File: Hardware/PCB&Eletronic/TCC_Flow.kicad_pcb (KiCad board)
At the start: 2 copper layers, 147.3 x 68.6 mm, 42 parts, among them J1 ESP01, M3 MountingHole_3.2mm_M3, Q1 BC337, Q2 BC337, Q3 BC337, Q4 BC337

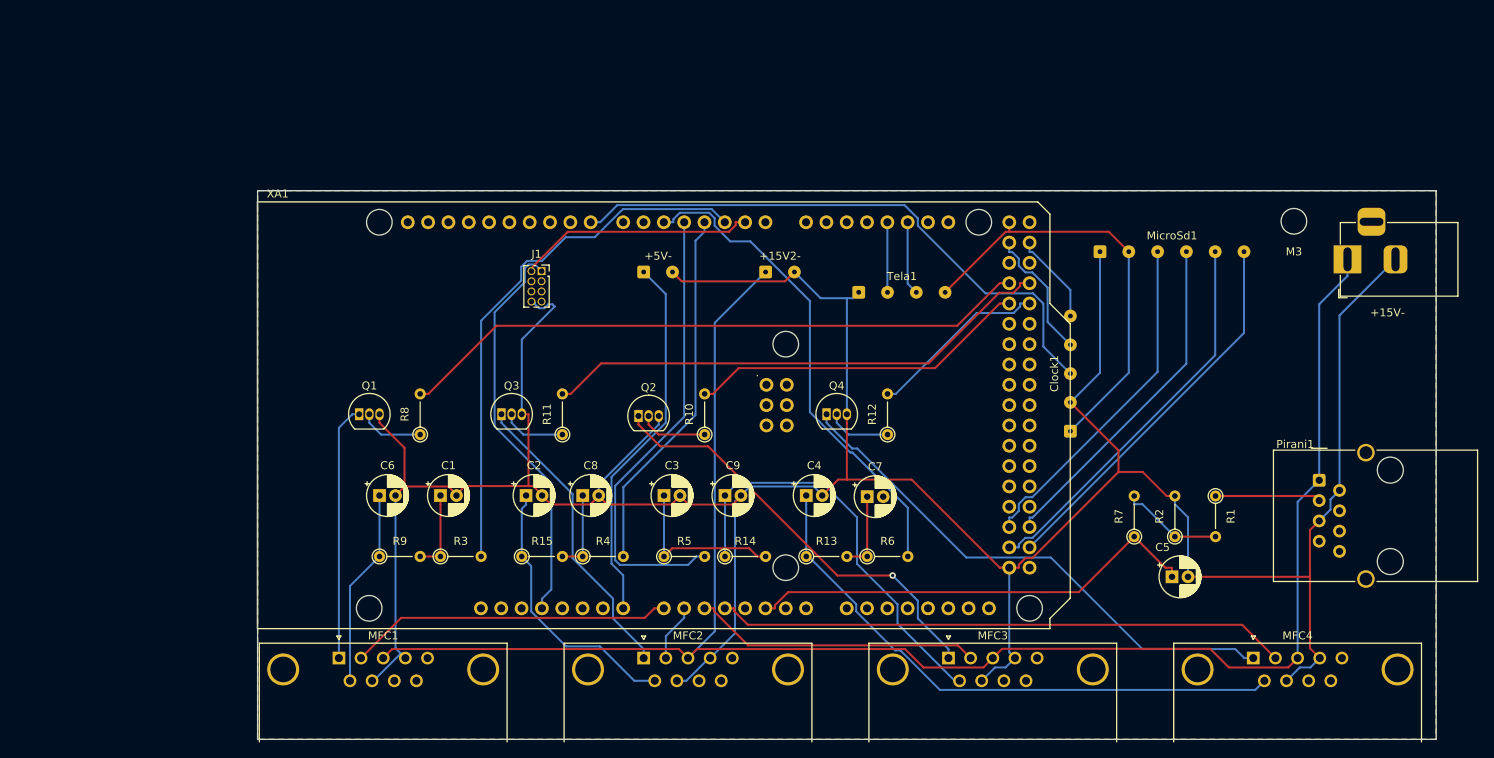
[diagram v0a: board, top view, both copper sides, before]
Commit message: [PCB] Add updated pcb and Doc
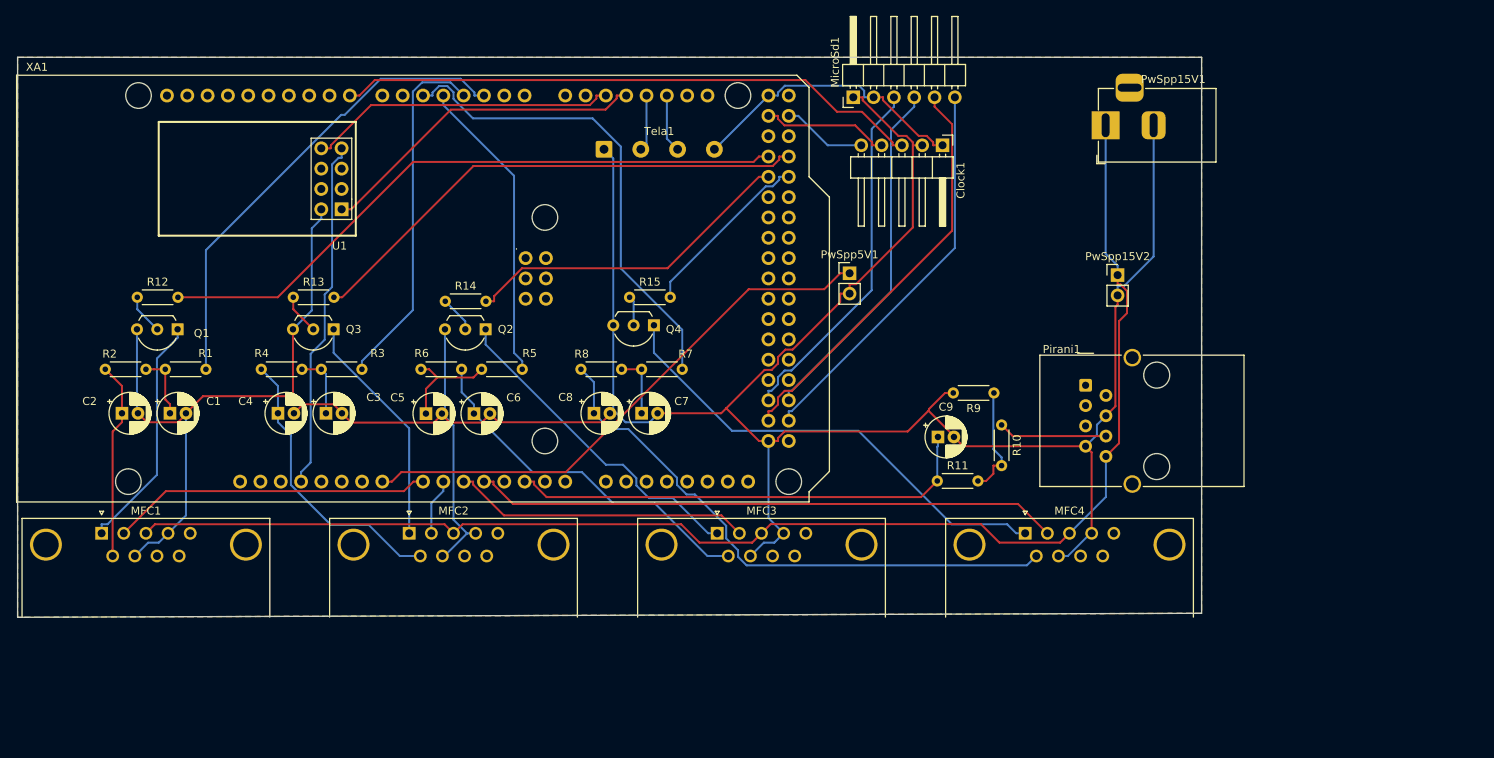
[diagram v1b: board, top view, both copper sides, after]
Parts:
- removed +15V-: Conn_01x02_Male, Connector_BarrelJack:BarrelJack_Horizontal
- removed +15V2-, +5V-: Conn_01x02_Male, Connector_Wire:SolderWire-0.1sqmm_1x02_P3.6mm_D0.4mm_OD1mm
- removed J1: ESP01, Connector_PinSocket_1.27mm:PinSocket_2x04_P1.27mm_Vertical
- removed M3: MountingHole_3.2mm_M3, MountingHole:MountingHole_3.2mm_M3
- added PwSpp15V1: Conn_01x02_Male, Connector_BarrelJack:BarrelJack_Horizontal, F.Cu at (169.5, 35.0)
- added PwSpp15V2: Conn_01x02_Male, Connector_PinHeader_2.54mm:PinHeader_1x02_P2.54mm_Vertical, F.Cu at (171.0, 53.7)
- added PwSpp5V1: Conn_01x02_Male, Connector_PinHeader_2.54mm:PinHeader_1x02_P2.54mm_Vertical, F.Cu at (137.5, 53.5)
- added U1: ESP-01v090, esp:ESP-01, F.Cu at (74.0, 45.5)
- Clock1: footprint Connector_Wire:SolderWire-0.1sqmm_1x05_P3.6mm_D0.4mm_OD1mm -> Connector_PinHeader_2.54mm:PinHeader_1x05_P2.54mm_Horizontal
- MicroSd1: footprint Connector_Wire:SolderWire-0.1sqmm_1x06_P3.6mm_D0.4mm_OD1mm -> Connector_PinHeader_2.54mm:PinHeader_1x06_P2.54mm_Horizontal
- Q1, Q2, Q3, Q4: footprint Package_TO_SOT_THT:TO-92_Inline -> Package_TO_SOT_THT:TO-92L_Inline_Wide
- R1, R2: value 4.6K -> 500; footprint Resistor_THT:R_Axial_DIN0204_L3.6mm_D1.6mm_P5.08mm_Vertical -> Resistor_THT:R_Axial_DIN0204_L3.6mm_D1.6mm_P5.08mm_Horizontal
- R10: value 4.7K -> 4.6K; footprint Resistor_THT:R_Axial_DIN0204_L3.6mm_D1.6mm_P5.08mm_Vertical -> Resistor_THT:R_Axial_DIN0204_L3.6mm_D1.6mm_P5.08mm_Horizontal
- R11: value 4.7K -> 220; footprint Resistor_THT:R_Axial_DIN0204_L3.6mm_D1.6mm_P5.08mm_Vertical -> Resistor_THT:R_Axial_DIN0204_L3.6mm_D1.6mm_P5.08mm_Horizontal
- R12: footprint Resistor_THT:R_Axial_DIN0204_L3.6mm_D1.6mm_P5.08mm_Vertical -> Resistor_THT:R_Axial_DIN0204_L3.6mm_D1.6mm_P5.08mm_Horizontal
- R13, R14, R15: value 1K -> 4.7K; footprint Resistor_THT:R_Axial_DIN0204_L3.6mm_D1.6mm_P5.08mm_Vertical -> Resistor_THT:R_Axial_DIN0204_L3.6mm_D1.6mm_P5.08mm_Horizontal
- R3, R4, R5, R6: value 1K -> 500; footprint Resistor_THT:R_Axial_DIN0204_L3.6mm_D1.6mm_P5.08mm_Vertical -> Resistor_THT:R_Axial_DIN0204_L3.6mm_D1.6mm_P5.08mm_Horizontal
- R7: value 220 -> 500; footprint Resistor_THT:R_Axial_DIN0204_L3.6mm_D1.6mm_P5.08mm_Vertical -> Resistor_THT:R_Axial_DIN0204_L3.6mm_D1.6mm_P5.08mm_Horizontal
- R8: value 4.7K -> 500; footprint Resistor_THT:R_Axial_DIN0204_L3.6mm_D1.6mm_P5.08mm_Vertical -> Resistor_THT:R_Axial_DIN0204_L3.6mm_D1.6mm_P5.08mm_Horizontal
- R9: value 1K -> 4.6K; footprint Resistor_THT:R_Axial_DIN0204_L3.6mm_D1.6mm_P5.08mm_Vertical -> Resistor_THT:R_Axial_DIN0204_L3.6mm_D1.6mm_P5.08mm_Horizontal
- Tela1: footprint Connector_Wire:SolderWire-0.1sqmm_1x04_P3.6mm_D0.4mm_OD1mm -> Connector_Wire:SolderWire-0.5sqmm_1x04_P4.6mm_D0.9mm_OD2.1mm
- moved R2 135.3 mm to (44.5, 65.5), turned to 0 degrees
- moved R1 132.2 mm to (52.0, 65.5), turned to 0 degrees
- moved C5 95.5 mm to (84.5, 71.0)
- moved R12 95.3 mm to (48.5, 56.5), turned to 0 degrees
- moved R9 79.5 mm to (155.5, 68.5), turned to 180 degrees
- moved R13 71.8 mm to (68.0, 56.5)
- moved C4 66.8 mm to (66.0, 71.0)
- moved R7 65.0 mm to (111.5, 65.5), turned to 0 degrees
- moved R6 55.8 mm to (89.0, 65.5), turned to 180 degrees
- moved C2 51.6 mm to (46.5, 71.0)
- moved R14 47.3 mm to (87.0, 57.0)
- moved R11 47.2 mm to (148.5, 79.5), turned to 0 degrees
- moved R4 46.5 mm to (64.0, 65.5)
- moved C3 43.5 mm to (72.0, 71.0)
- moved Clock1 39.1 mm to (149.1, 37.5), turned to -90 degrees
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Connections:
- C1 pad 1: Net-(R3-Pad1) -> Net-(C1-Pad1)
- C2 pad 1: Net-(MFC2-Pad6) -> Net-(C2-Pad1)
- C3 pad 1: Net-(R5-Pad1) -> Net-(C3-Pad1)
- C4 pad 1: Net-(MFC4-Pad6) -> Net-(C4-Pad1)
- C7 pad 1: Net-(R6-Pad1) -> Net-(C7-Pad1)
- C7 pad 2: unconnected-(C7-Pad2) -> Net-(C1-Pad2)
- C8 pad 1: Net-(R4-Pad1) -> Net-(C8-Pad1)
- C9 pad 1: Net-(MFC3-Pad6) -> Net-(C9-Pad1)
- MFC1 pad 6: Net-(C6-Pad1) -> Net-(C2-Pad1)
- MFC2 pad 6: Net-(MFC2-Pad6) -> Net-(C4-Pad1)
- MFC3 pad 6: Net-(MFC3-Pad6) -> Net-(C6-Pad1)
- MFC4 pad 6: Net-(MFC4-Pad6) -> Net-(C8-Pad1)
- Pirani1 pad 1: Net-(MFC1-Pad3) -> unconnected-(Pirani1-Pad1)
- Pirani1 pad 2: Net-(C1-Pad2) -> unconnected-(Pirani1-Pad2)
- Pirani1 pad 3: Net-(Pirani1-Pad3) -> unconnected-(Pirani1-Pad3)
- Pirani1 pad 4: unconnected-(Pirani1-Pad4) -> Net-(C1-Pad2)
- Pirani1 pad 5: Net-(C1-Pad2) -> unconnected-(Pirani1-Pad5)
- Pirani1 pad 6: unconnected-(Pirani1-Pad6) -> Net-(Pirani1-Pad6)
- Pirani1 pad 7: unconnected-(Pirani1-Pad7) -> Net-(C1-Pad2)
- Pirani1 pad 8: unconnected-(Pirani1-Pad8) -> Net-(MFC1-Pad3)
- R1 pad 1: Net-(Pirani1-Pad3) -> Net-(C1-Pad1)
- R10 pad 1: Net-(Q2-Pad2) -> Net-(Pirani1-Pad6)
- R11 pad 1: Net-(Q3-Pad2) -> Net-(C9-Pad1)
- R11 pad 2: Net-(R11-Pad2) -> Net-(R10-Pad2)
- R12 pad 1: Net-(Q4-Pad2) -> Net-(Q1-Pad2)
- R12 pad 2: Net-(XA1-PadD29) -> Net-(R12-Pad2)
- R13 pad 1: Net-(MFC4-Pad6) -> Net-(Q3-Pad2)
- R13 pad 2: Net-(R6-Pad1) -> Net-(R13-Pad2)
- R14 pad 1: Net-(MFC3-Pad6) -> Net-(Q2-Pad2)
- R14 pad 2: Net-(R5-Pad1) -> Net-(R14-Pad2)
- R15 pad 1: Net-(MFC2-Pad6) -> Net-(Q4-Pad2)
- R15 pad 2: Net-(R4-Pad1) -> Net-(R15-Pad2)
- R2 pad 1: Net-(R1-Pad2) -> Net-(C2-Pad1)
- R2 pad 2: Net-(C1-Pad2) -> Net-(C1-Pad1)
- R3 pad 1: Net-(R3-Pad1) -> Net-(C3-Pad1)
- R4 pad 1: Net-(R4-Pad1) -> Net-(C4-Pad1)
- R4 pad 2: Net-(R4-Pad2) -> Net-(C3-Pad1)
- R5 pad 1: Net-(R5-Pad1) -> Net-(C5-Pad1)
- R6 pad 1: Net-(R6-Pad1) -> Net-(C6-Pad1)
- R6 pad 2: Net-(R6-Pad2) -> Net-(C5-Pad1)
- R7 pad 1: Net-(C5-Pad1) -> Net-(C7-Pad1)
- R7 pad 2: Net-(R1-Pad2) -> Net-(R7-Pad2)
- R8 pad 1: Net-(Q1-Pad2) -> Net-(C8-Pad1)
- R8 pad 2: Net-(R8-Pad2) -> Net-(C7-Pad1)
- R9 pad 1: Net-(C6-Pad1) -> Net-(R10-Pad2)
- R9 pad 2: Net-(R3-Pad1) -> Net-(C1-Pad2)
- XA1 pad A5: Net-(C5-Pad1) -> Net-(C9-Pad1)
- XA1 pad D1: Net-(XA1-PadD1) -> unconnected-(XA1-PadD1)
- XA1 pad D16: unconnected-(XA1-PadD16) -> Net-(U1-Pad8)
- XA1 pad D17: unconnected-(XA1-PadD17) -> Net-(U1-Pad1)
- XA1 pad D2: Net-(R3-Pad2) -> Net-(R1-Pad2)
- XA1 pad D26: Net-(R8-Pad2) -> Net-(R12-Pad2)
- XA1 pad D27: Net-(R11-Pad2) -> Net-(R13-Pad2)
- XA1 pad D28: Net-(R10-Pad2) -> Net-(R14-Pad2)
- XA1 pad D29: Net-(XA1-PadD29) -> Net-(R15-Pad2)
- XA1 pad D3: Net-(R4-Pad2) -> Net-(R3-Pad2)
- XA1 pad D5: Net-(R6-Pad2) -> Net-(R7-Pad2)
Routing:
- net Net-(R12-Pad2): track 0.00 -> 81.1 mm
- net Net-(R8-Pad2): track 79.4 -> 0.00 mm
- net Net-(MFC4-Pad6): track 72.8 -> 0.00 mm
- net Net-(C8-Pad1): track 0.00 -> 71.8 mm
- net Net-(R13-Pad2): track 0.00 -> 64.4 mm
- net Net-(R11-Pad2): track 64.4 -> 0.00 mm
- net Net-(R6-Pad2): track 61.3 -> 0.00 mm
- net Net-(R7-Pad2): track 0.00 -> 60.1 mm
- net Net-(C9-Pad1): track 0.00 -> 59.0 mm
- net Net-(MFC3-Pad6): track 52.7 -> 0.00 mm
- net Net-(MFC1-Pad3): track 223.8 -> 175.5 mm
- net Net-(R1-Pad2): track 12.9 -> 59.6 mm
- net Net-(R4-Pad2): track 46.0 -> 0.00 mm
- net Net-(C5-Pad1): track 57.5 -> 13.5 mm
- net Net-(R14-Pad2): track 0.00 -> 42.1 mm
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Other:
- board size 147.3 x 68.6 mm -> 148 x 70 mm
